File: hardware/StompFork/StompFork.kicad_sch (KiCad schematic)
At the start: 32 parts, among them J1 Line-Level Input, J2 Direct Output, J3 Stompbox Output 1, J4 Stompbox Output 2, J5 Power, U1 TL074

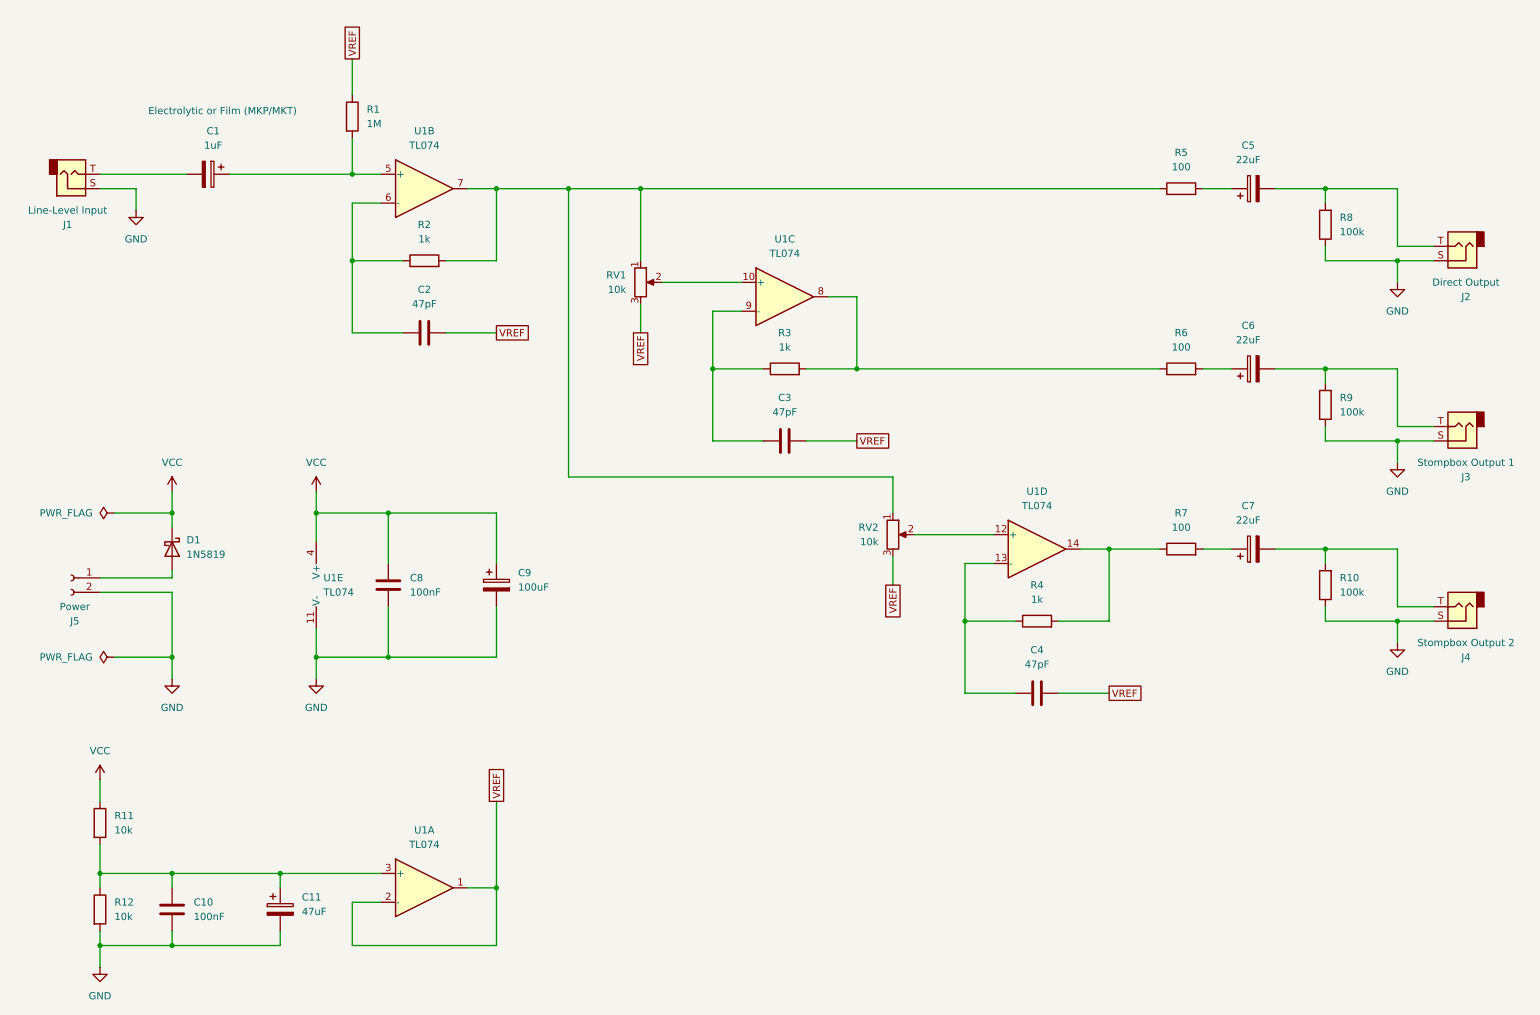
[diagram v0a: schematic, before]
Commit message: Update PCB
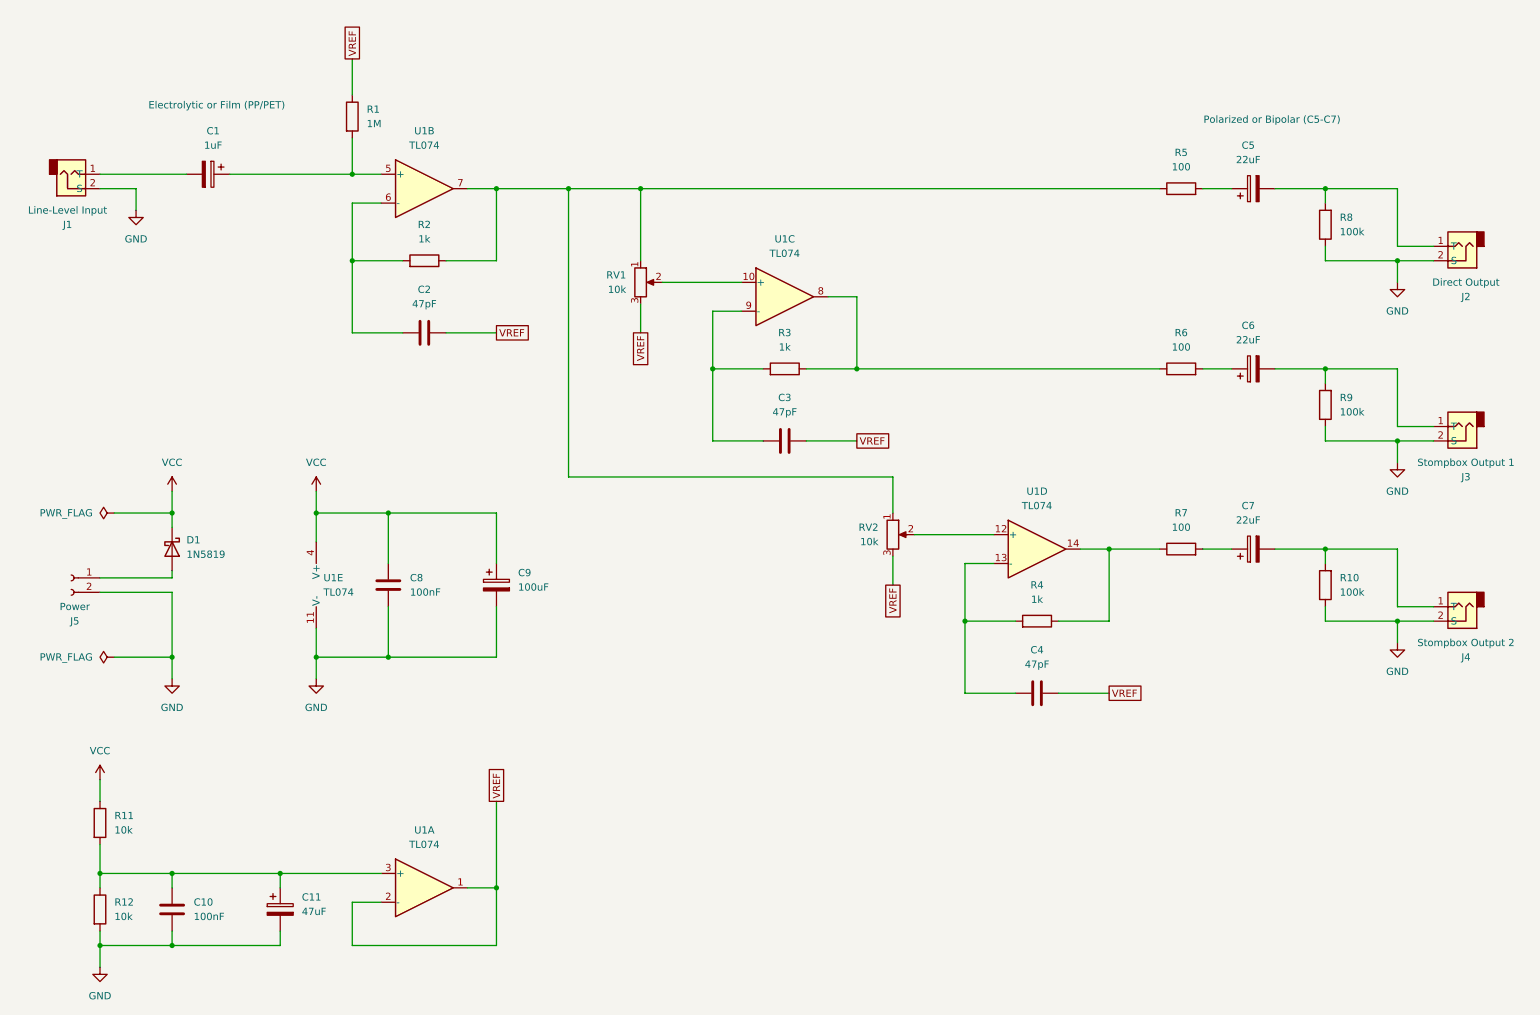
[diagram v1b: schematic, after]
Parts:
- C1: footprint (none) -> Capacitor_THT:C_Rect_L24.0mm_W7.0mm_P22.50mm_MKT
- C10, C2, C3, C4, C8: footprint (none) -> Capacitor_THT:C_Disc_D5.0mm_W2.5mm_P5.00mm
- C11, C9: footprint (none) -> Capacitor_THT:C_Radial_D6.3mm_H11.0mm_P2.50mm
- C5, C6, C7: footprint (none) -> Capacitor_THT:C_Radial_D10.0mm_H12.5mm_P5.00mm
- J1, J2, J3, J4, J5: footprint (none) -> Connector_JST:JST_EH_B2B-EH-A_1x02_P2.50mm_Vertical
- R1, R2, R3, R4: footprint (none) -> Resistor_THT:R_Axial_DIN0207_L6.3mm_D2.5mm_P2.54mm_Vertical
- R10, R11, R12, R5, R6, R7, R8, R9: footprint (none) -> Resistor_THT:R_Axial_DIN0207_L6.3mm_D2.5mm_P10.16mm_Horizontal
- RV1, RV2: footprint (none) -> Connector_JST:JST_EH_B3B-EH-A_1x03_P2.50mm_Vertical
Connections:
- net GND: now also J1.2 (S), J2.2 (S), J3.2 (S), J4.2 (S); no longer J1.S, J2.S, J3.S, J4.S
- net at C4.1, U1.13 (-): now also R4.2; no longer R4.1
- net at R7.1, U1.14: now also R4.1; no longer R4.2
- net at C2.1, U1.6 (-): now also R2.2; no longer R2.1
- net at R5.1, RV1.1, RV2.1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: now also R2.1; no longer R2.2
- net at C1.2: now also J1.1 (T); no longer J1.T
- net at C3.1, U1.9 (-): now also R3.2; no longer R3.1
- net at R6.1, U1.8: now also R3.1; no longer R3.2
- net at C7.2, R10.2: now also J4.1 (T); no longer J4.T
- net at C6.2, R9.2: now also J3.1 (T); no longer J3.T
- net at C5.2, R8.2: now also J2.1 (T); no longer J2.T
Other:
- moved on the sheet: R2, R3, R4
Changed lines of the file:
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@@
 	(symbol
 		(lib_id "Device:R")
-		(at 196.85 120.65 90)
+		(at 196.85 120.65 270)
+		(mirror x)
 		(unit 1)
 		(exclude_from_sim no)
@@
 			)
 		)
-		(property "Footprint" ""
+		(property "Footprint" "Resistor_THT:R_Axial_DIN0207_L6.3mm_D2.5mm_P2.54mm_Vertical"
 			(at 196.85 122.428 90)
 			(effects
@@
 	(symbol
 		(lib_id "Device:R")
-		(at 88.9 57.15 90)
+		(at 88.9 57.15 270)
+		(mirror x)
 		(unit 1)
 		(exclude_from_sim no)
@@
 			)
 		)
-		(property "Footprint" ""
+		(property "Footprint" "Resistor_THT:R_Axial_DIN0207_L6.3mm_D2.5mm_P2.54mm_Vertical"
 			(at 88.9 58.928 90)
 			(effects
@@
 			)
 		)
-		(property "Footprint" ""
+		(property "Footprint" "Resistor_THT:R_Axial_DIN0207_L6.3mm_D2.5mm_P2.54mm_Vertical"
 			(at 74.422 31.75 90)
 			(effects
@@
 			)
 		)
-		(property "Footprint" ""
+		(property "Footprint" "Capacitor_THT:C_Rect_L24.0mm_W7.0mm_P22.50mm_MKT"
 			(at 46.99 42.8752 0)
 			(effects
@@
 			)
 		)
-		(property "Description" "Electrolytic or Film (MKP/MKT)"
-			(at 53.34 30.734 90)
+		(property "Description" "Electrolytic or Film (PP/PET)"
+			(at 52.324 29.718 90)
 			(effects
 				(font
@@
 	(symbol
 		(lib_id "Device:R")
-		(at 152.4 76.2 90)
+		(at 152.4 76.2 270)
+		(mirror x)
 		(unit 1)
 		(exclude_from_sim no)
@@
 			)
 		)
-		(property "Footprint" ""
+		(property "Footprint" "Resistor_THT:R_Axial_DIN0207_L6.3mm_D2.5mm_P2.54mm_Vertical"
 			(at 152.4 77.978 90)
 			(effects
@@
 			)
 		)
-		(property "Footprint" ""
+		(property "Footprint" "Capacitor_THT:C_Disc_D5.0mm_W2.5mm_P5.00mm"
 			(at 200.66 134.3152 0)
 			(effects
@@
 			)
 		)
-		(property "Footprint" ""
+		(property "Footprint" "Resistor_THT:R_Axial_DIN0207_L6.3mm_D2.5mm_P10.16mm_Horizontal"
 			(at 222.25 46.228 90)
 			(effects
@@
 			)
 		)
-		(property "Footprint" ""
+		(property "Footprint" "Connector_JST:JST_EH_B2B-EH-A_1x02_P2.50mm_Vertical"
 			(at 271.78 118.11 0)
 			(effects
@@
 			)
 		)
-		(pin "T"
+		(pin "2"
 		)
-		(pin "S"
+		(pin "1"
 		)
 		(instances
@@
 			)
 		)
-		(property "Footprint" ""
+		(property "Footprint" "Capacitor_THT:C_Radial_D6.3mm_H11.0mm_P2.50mm"
 			(at 102.5652 118.11 0)
 			(effects
@@
 			)
 		)
-		(property "Footprint" ""
+		(property "Footprint" "Capacitor_THT:C_Radial_D6.3mm_H11.0mm_P2.50mm"
 			(at 64.4652 175.26 0)
 			(effects
@@
 	)
 	(symbol
+		(lib_name "AudioJack2_1")
 		(lib_id "Connector_Audio:AudioJack2")
 		(at 26.67 41.91 0)
@@
 			)
 		)
-		(property "Footprint" ""
+		(property "Footprint" "Connector_JST:JST_EH_B2B-EH-A_1x02_P2.50mm_Vertical"
 			(at 26.67 41.91 0)
 			(effects
@@
 			)
 		)
-		(pin "T"
+		(pin "2"
 		)
-		(pin "S"
+		(pin "1"
 		)
 		(instances
@@
 			)
 		)
-		(property "Footprint" ""
+		(property "Footprint" "Capacitor_THT:C_Disc_D5.0mm_W2.5mm_P5.00mm"
 			(at 45.4152 175.26 0)
 			(effects
@@
 			)
 		)
-		(property "Footprint" ""
+		(property "Footprint" "Capacitor_THT:C_Radial_D10.0mm_H12.5mm_P5.00mm"
 			(at 238.76 106.9848 0)
 			(effects
@@
 			)
 		)
-		(property "Footprint" ""
+		(property "Footprint" "Resistor_THT:R_Axial_DIN0207_L6.3mm_D2.5mm_P10.16mm_Horizontal"
 			(at 222.25 109.728 90)
 			(effects
@@
 			)
 		)
-		(property "Footprint" ""
+		(property "Footprint" "Resistor_THT:R_Axial_DIN0207_L6.3mm_D2.5mm_P10.16mm_Horizontal"
 			(at 249.428 82.55 90)
 			(effects
@@
 			)
 		)
-		(property "Footprint" ""
+		(property "Footprint" "Capacitor_THT:C_Disc_D5.0mm_W2.5mm_P5.00mm"
 			(at 83.5152 118.11 0)
 			(effects
@@
 			)
 		)
-		(property "Footprint" ""
+		(property "Footprint" "Resistor_THT:R_Axial_DIN0207_L6.3mm_D2.5mm_P10.16mm_Horizontal"
 			(at 249.428 114.3 90)
 			(effects
@@
 	)
 	(symbol
+		(lib_name "AudioJack2_3")
 		(lib_id "Connector_Audio:AudioJack2")
 		(at 271.78 86.36 180)
@@
 			)
 		)
-		(property "Footprint" ""
+		(property "Footprint" "Connector_JST:JST_EH_B2B-EH-A_1x02_P2.50mm_Vertical"
 			(at 271.78 86.36 0)
 			(effects
@@
 			)
 		)
-		(pin "T"
+		(pin "2"
 		)
-		(pin "S"
+		(pin "1"
 		)
 		(instances
@@
 			)
 		)
-		(property "Footprint" ""
+		(property "Footprint" "Resistor_THT:R_Axial_DIN0207_L6.3mm_D2.5mm_P10.16mm_Horizontal"
 			(at 29.972 156.21 90)
 			(effects
@@
 		(on_board yes)
 		(dnp no)
-		(fields_autoplaced yes)
 		(property "Reference" "C5"
 			(at 234.061 36.83 90)
@@
 			)
 		)
-		(property "Footprint" ""
+		(property "Footprint" "Capacitor_THT:C_Radial_D10.0mm_H12.5mm_P5.00mm"
 			(at 238.76 43.4848 0)
 			(effects
@@
 			)
 		)
-		(property "Description" "Polarized capacitor"
-			(at 234.95 44.45 0)
+		(property "Description" "Polarized or Bipolar (C5-C7)"
+			(at 238.252 32.258 90)
 			(effects
 				(font
 					(size 1.27 1.27)
 				)
-				(hide yes)
 			)
 		)
@@
 			)
 		)
-		(property "Footprint" ""
+		(property "Footprint" "Connector_JST:JST_EH_B3B-EH-A_1x03_P2.50mm_Vertical"
 			(at 171.45 105.41 0)
 			(effects
@@
 	)
 	(symbol
+		(lib_name "AudioJack2_2")
 		(lib_id "Connector_Audio:AudioJack2")
 		(at 271.78 54.61 180)
@@
 			)
 		)
-		(property "Footprint" ""
+		(property "Footprint" "Connector_JST:JST_EH_B2B-EH-A_1x02_P2.50mm_Vertical"
 			(at 271.78 54.61 0)
 			(effects
@@
 			)
 		)
-		(pin "T"
+		(pin "2"
 		)
-		(pin "S"
+		(pin "1"
 		)
 		(instances
@@
 			)
 		)
-		(property "Footprint" ""
+		(property "Footprint" "Capacitor_THT:C_Disc_D5.0mm_W2.5mm_P5.00mm"
 			(at 156.21 89.8652 0)
 			(effects
@@
 			)
 		)
-		(property "Footprint" ""
+		(property "Footprint" "Connector_JST:JST_EH_B2B-EH-A_1x02_P2.50mm_Vertical"
 			(at 26.67 113.03 0)
 			(effects
@@
 			)
 		)
-		(property "Footprint" ""
+		(property "Footprint" "Capacitor_THT:C_Radial_D10.0mm_H12.5mm_P5.00mm"
 			(at 238.76 75.2348 0)
 			(effects
@@
 			)
 		)
-		(property "Footprint" ""
+		(property "Footprint" "Capacitor_THT:C_Disc_D5.0mm_W2.5mm_P5.00mm"
 			(at 92.71 70.8152 0)
 			(effects
@@
 			)
 		)
-		(property "Footprint" ""
+		(property "Footprint" "Resistor_THT:R_Axial_DIN0207_L6.3mm_D2.5mm_P10.16mm_Horizontal"
 			(at 222.25 77.978 90)
 			(effects
@@
 			)
 		)
-		(property "Footprint" ""
+		(property "Footprint" "Connector_JST:JST_EH_B3B-EH-A_1x03_P2.50mm_Vertical"
 			(at 127 60.96 0)
 			(effects
@@
 			)
 		)
-		(property "Footprint" ""
+		(property "Footprint" "Resistor_THT:R_Axial_DIN0207_L6.3mm_D2.5mm_P10.16mm_Horizontal"
 			(at 29.972 171.45 90)
 			(effects
@@
 			)
 		)
-		(property "Footprint" ""
+		(property "Footprint" "Resistor_THT:R_Axial_DIN0207_L6.3mm_D2.5mm_P10.16mm_Horizontal"
 			(at 249.428 50.8 90)
 			(effects
